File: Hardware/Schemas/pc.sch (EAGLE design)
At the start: 4 parts

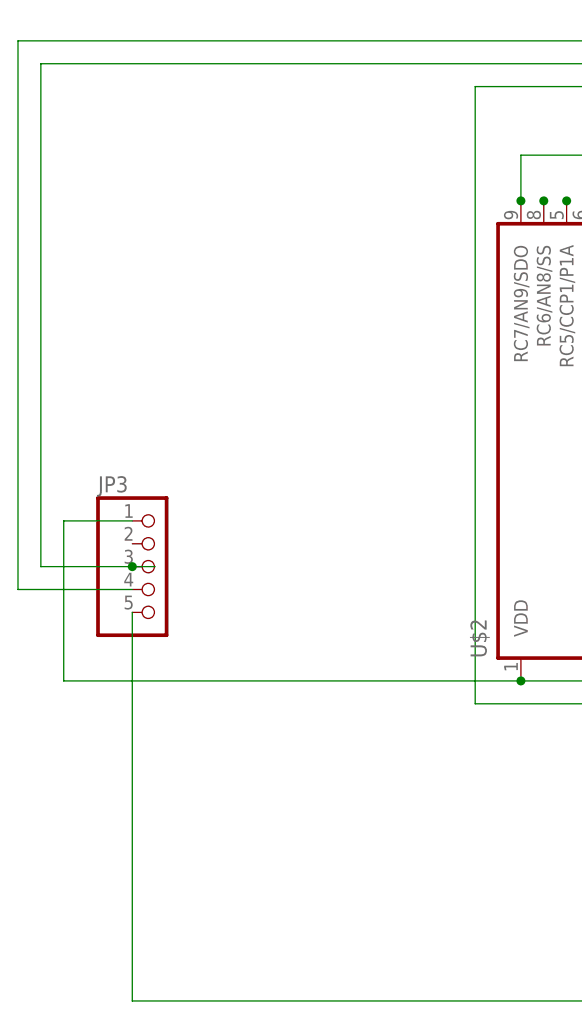
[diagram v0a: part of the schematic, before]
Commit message: a
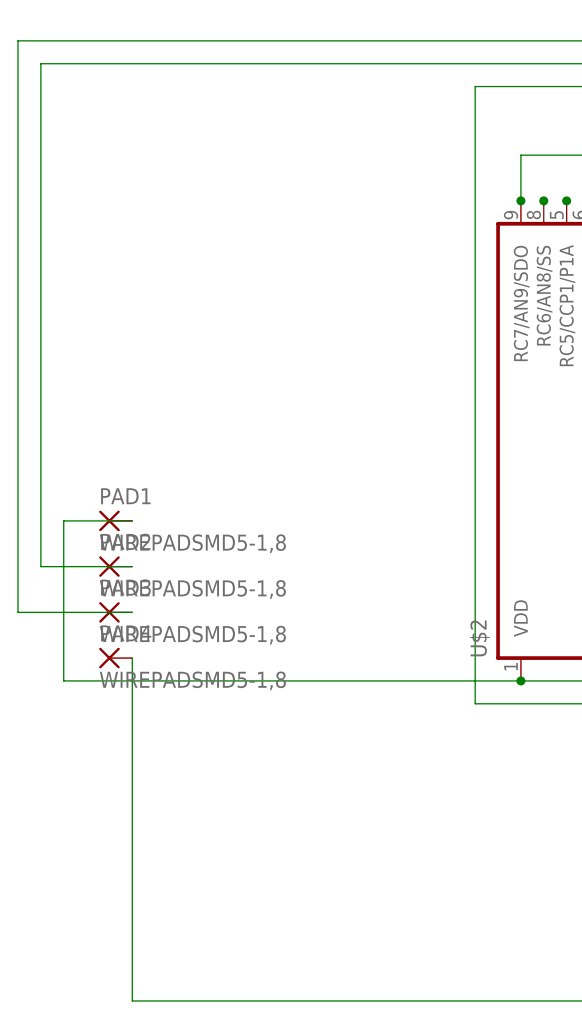
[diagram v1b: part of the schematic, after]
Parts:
- removed JP3: (no value), pinhead:PINHD-1X5/90
- added PAD1, PAD2, PAD3, PAD4: WIREPADSMD5-1,8, wirepad:WIREPADSMD5-1,8
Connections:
- net N$17: now also PAD1.P; no longer JP3.1
- net N$33: now also PAD3.P; no longer JP3.4
- net N$34: now also PAD2.P; no longer JP3.3
- net N$5: now also PAD4.P; no longer JP3.5
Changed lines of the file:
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@@
 <part name="U$2" library="microchip" deviceset="PIC16F690*" device=""/>
 <part name="JP2" library="pinhead" deviceset="PINHD-1X5" device="" value="Prog"/>
-<part name="JP3" library="pinhead" deviceset="PINHD-1X5" device="/90"/>
+<part name="PAD1" library="wirepad" deviceset="WIREPAD" device="SMD5-1,8"/>
+<part name="PAD2" library="wirepad" deviceset="WIREPAD" device="SMD5-1,8"/>
+<part name="PAD3" library="wirepad" deviceset="WIREPAD" device="SMD5-1,8"/>
+<part name="PAD4" library="wirepad" deviceset="WIREPAD" device="SMD5-1,8"/>
 </parts>
 <sheets>
@@
 <instance part="U$2" gate="G$1" x="134.62" y="68.58" rot="R90"/>
 <instance part="JP2" gate="A" x="162.56" y="121.92"/>
-<instance part="JP3" gate="A" x="43.18" y="78.74"/>
+<instance part="PAD1" gate="G$1" x="38.1" y="83.82"/>
+<instance part="PAD2" gate="G$1" x="38.1" y="78.74"/>
+<instance part="PAD3" gate="G$1" x="38.1" y="73.66"/>
+<instance part="PAD4" gate="G$1" x="38.1" y="68.58"/>
 </instances>
 <busses>
@@
 <junction x="132.08" y="30.48"/>
 <pinref part="JP2" gate="A" pin="3"/>
-<pinref part="JP3" gate="A" pin="5"/>
-<wire x1="40.64" y1="73.66" x2="40.64" y2="30.48" width="0.1524" layer="91"/>
+<wire x1="40.64" y1="68.58" x2="40.64" y2="30.48" width="0.1524" layer="91"/>
+<pinref part="PAD4" gate="G$1" pin="P"/>
 </segment>
 </net>
@@
 <wire x1="33.02" y1="66.04" x2="83.82" y2="66.04" width="0.1524" layer="91"/>
 <junction x="83.82" y="66.04"/>
-<pinref part="JP3" gate="A" pin="1"/>
 <wire x1="40.64" y1="83.82" x2="33.02" y2="83.82" width="0.1524" layer="91"/>
+<pinref part="PAD1" gate="G$1" pin="P"/>
 </segment>
 </net>
@@
 <wire x1="27.94" y1="137.16" x2="106.68" y2="137.16" width="0.1524" layer="91"/>
 <wire x1="106.68" y1="137.16" x2="106.68" y2="119.38" width="0.1524" layer="91"/>
-<pinref part="JP3" gate="A" pin="4"/>
-<wire x1="40.64" y1="76.2" x2="27.94" y2="76.2" width="0.1524" layer="91"/>
-<wire x1="27.94" y1="76.2" x2="27.94" y2="137.16" width="0.1524" layer="91"/>
+<wire x1="40.64" y1="73.66" x2="27.94" y2="73.66" width="0.1524" layer="91"/>
+<wire x1="27.94" y1="73.66" x2="27.94" y2="137.16" width="0.1524" layer="91"/>
+<pinref part="PAD3" gate="G$1" pin="P"/>
 </segment>
 </net>
@@
 <wire x1="30.48" y1="134.62" x2="30.48" y2="78.74" width="0.1524" layer="91"/>
 <wire x1="30.48" y1="78.74" x2="40.64" y2="78.74" width="0.1524" layer="91"/>
-<pinref part="JP3" gate="A" pin="3"/>
-<wire x1="40.64" y1="78.74" x2="43.18" y2="78.74" width="0.1524" layer="91"/>
-<junction x="40.64" y="78.74"/>
-</segment>
-</net>
+<pinref part="PAD2" gate="G$1" pin="P"/>
+</segment>
+</net>
